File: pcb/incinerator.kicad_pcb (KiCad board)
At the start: 2 copper layers, 73.7 x 76.8 mm, 51 parts, among them J1 Power Source 12V, J2 IGNITION_MAIN, J3 IGNITION_AFT, J4 VALVE_MAIN, J5 VALVE_AFT_HI, J6 VALVE_AFT_LO, J7 AIRPMP, J8 To encoder, J9 To e-paper, Q1 IRLU120N, Q2 IRLU120N, Q3 IRLU120N, Q4 IRLU120N, Q5 IRLU120N, Q6 IRLU120N, U1 R-7890-0.5, U2 NodeMCU_ESP32, U3 Adafruit MAX31855, U4 Adafruit MAX31855

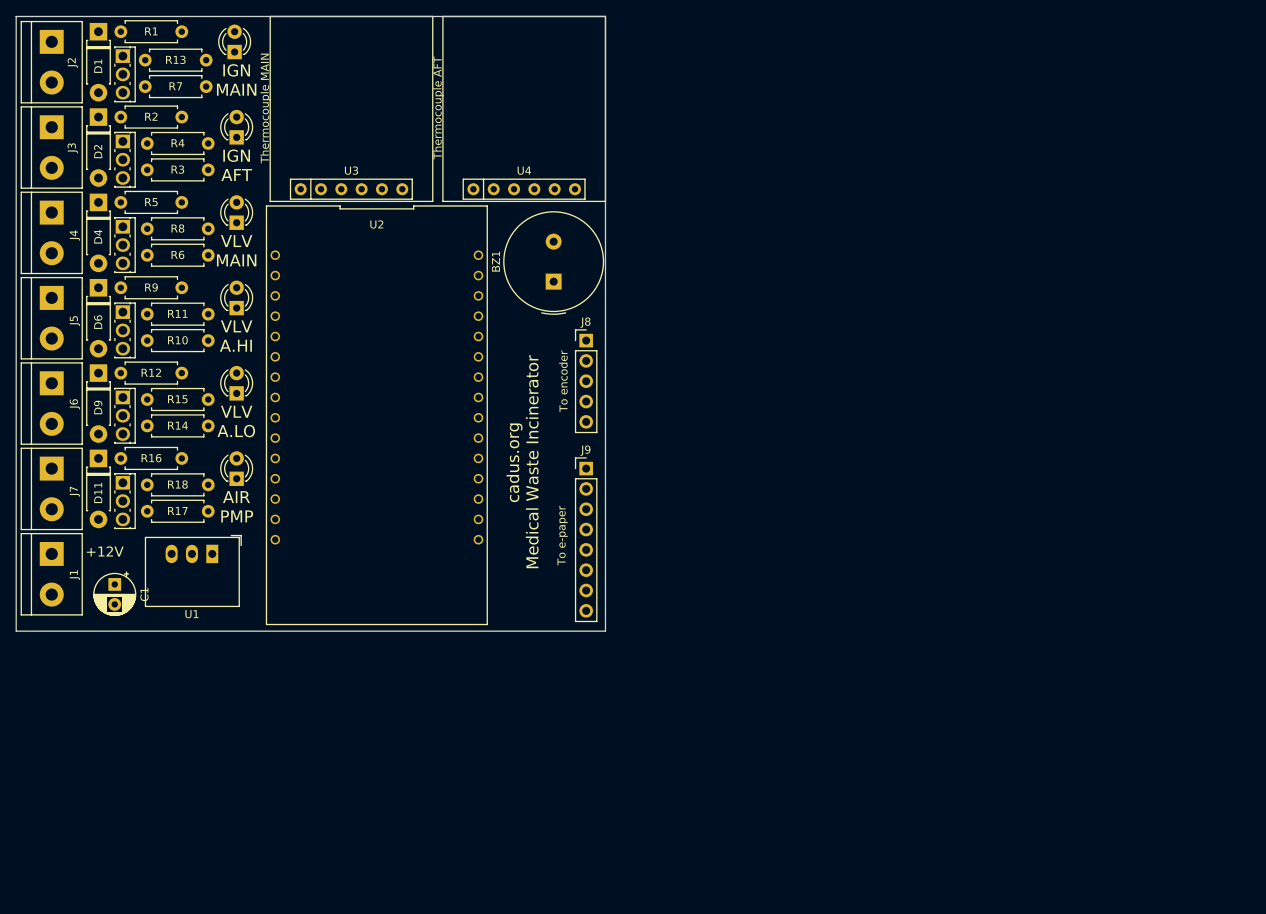
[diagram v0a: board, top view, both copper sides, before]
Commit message: Add PCB infos
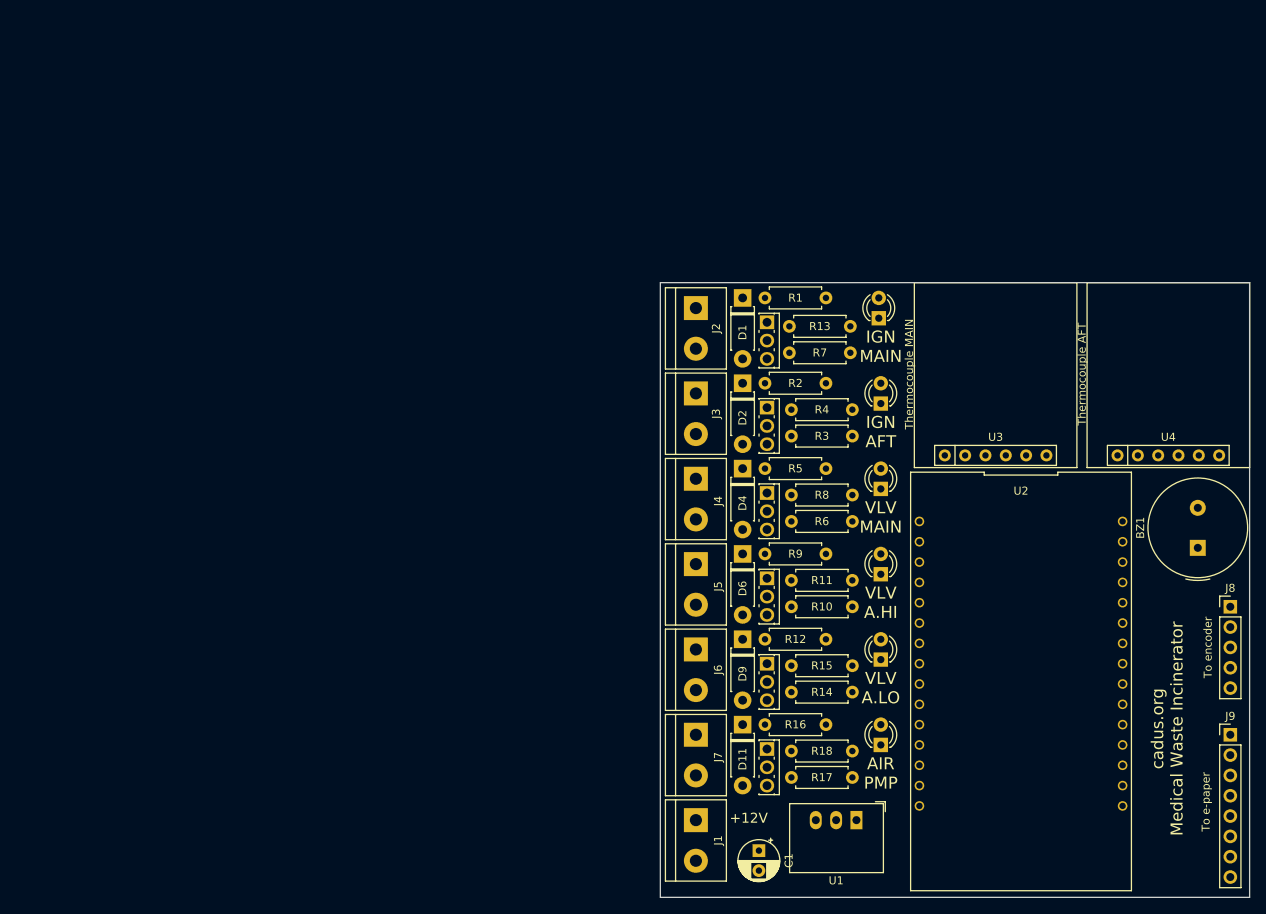
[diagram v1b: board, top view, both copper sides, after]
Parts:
- moved BZ1 87.1 mm to (168.7, 83.6)
- moved C1 87.1 mm to (113.8, 121.4)
- moved D1 87.1 mm to (111.8, 52.3)
- moved D10 87.1 mm to (129.0, 97.5)
- moved D11 87.1 mm to (111.8, 105.7)
- moved D12 87.1 mm to (129.0, 108.2)
- moved D2 87.1 mm to (111.8, 63.0)
- moved D3 87.1 mm to (129.0, 65.5)
- moved D4 87.1 mm to (111.8, 73.7)
- moved D5 87.1 mm to (129.0, 76.2)
- moved D6 87.1 mm to (111.8, 84.3)
- moved D7 87.1 mm to (128.8, 54.9)
- moved D8 87.1 mm to (129.0, 86.9)
- moved D9 87.1 mm to (111.8, 95.0)
- moved J1 87.1 mm to (105.9, 117.6)
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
